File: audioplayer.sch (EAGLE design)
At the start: 28 parts, among them J1 MICRO-SDCARD-CONNECTOR-330006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, J10 CONNECTOR-HEADER-8P-3460290P1, J11 CONNECTOR-HEADER-8P-3460290P1, J2 JST-2P-SMD-PW-3410050P1, J3 MICRO-USB-5P-340015001, J4 CONNECTOR-HEADER-2X3P-3460180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, J5 AUDIO-CONNECTOR-6P-SMD-344003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, J6 SCREW-TERMINAL-2P-3470070P1, J7 CONNECTOR-HEADER-6P-3460650P1, J8 CONNECTOR-HEADER-6P-3460270P1, J9 CONNECTOR-HEADER-10P-3460170P1, K1 BUTTON-4P-3100010P1, U1 ATMEGA328P-AU-1030060P1, U2 CN3065-1320040P1, U3 XC6206-3.3-1300260P1, X1 CRYSTAL-0500290P1

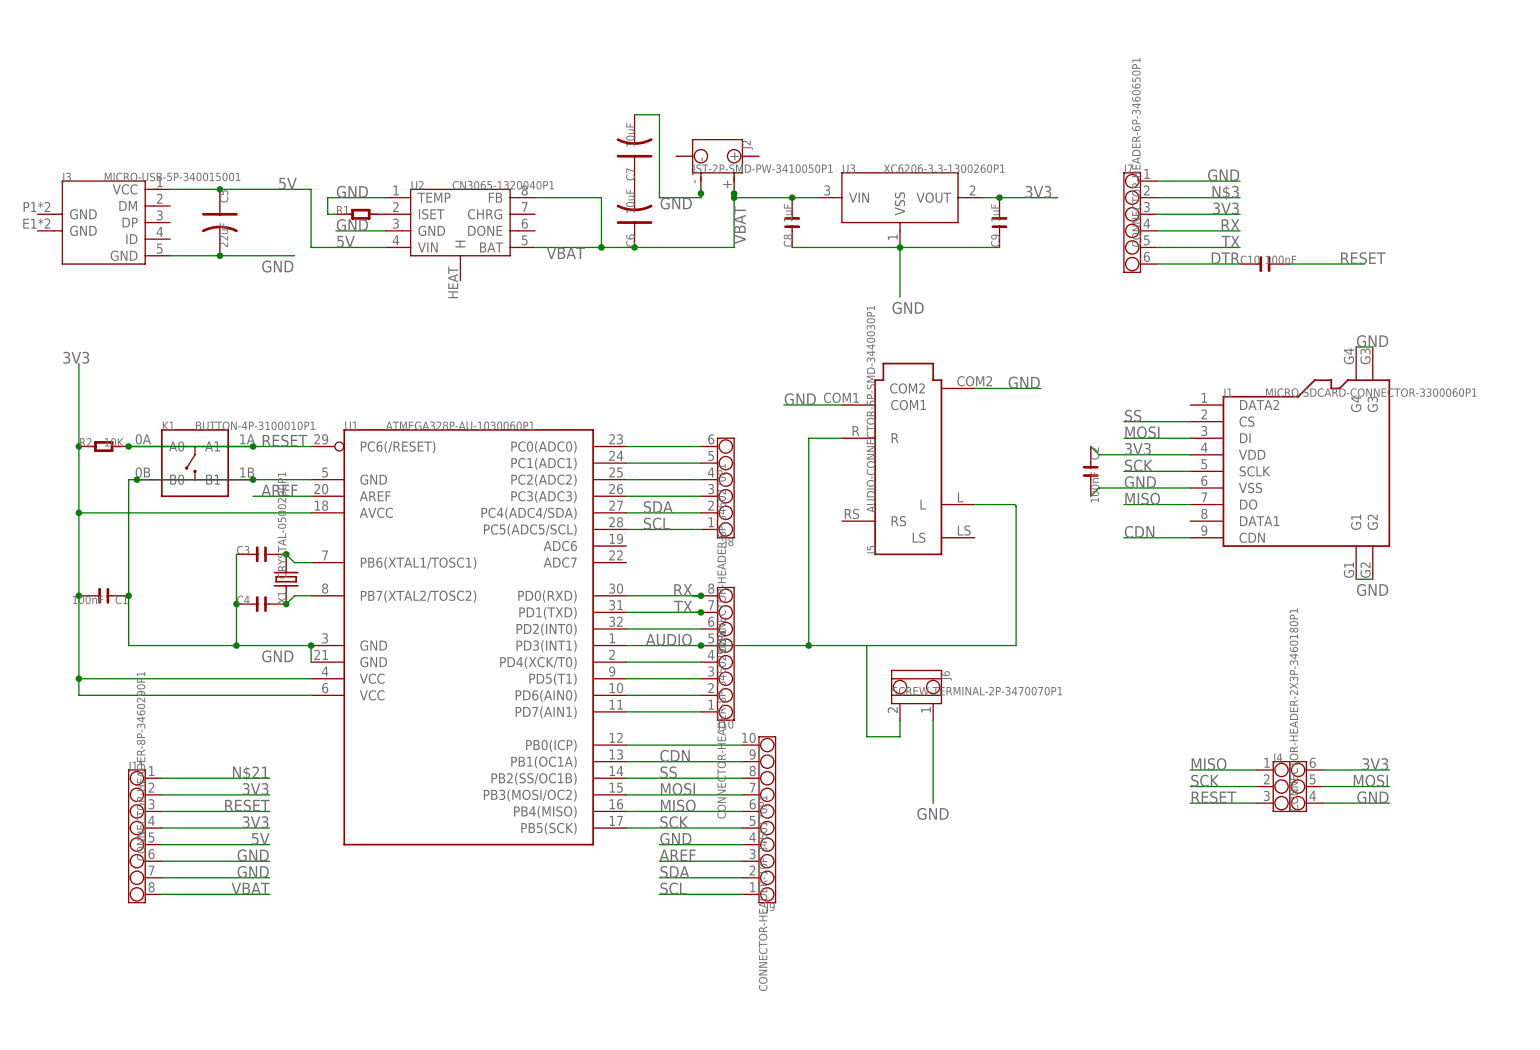
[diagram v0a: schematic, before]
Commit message: 1.5 hrs: routing.
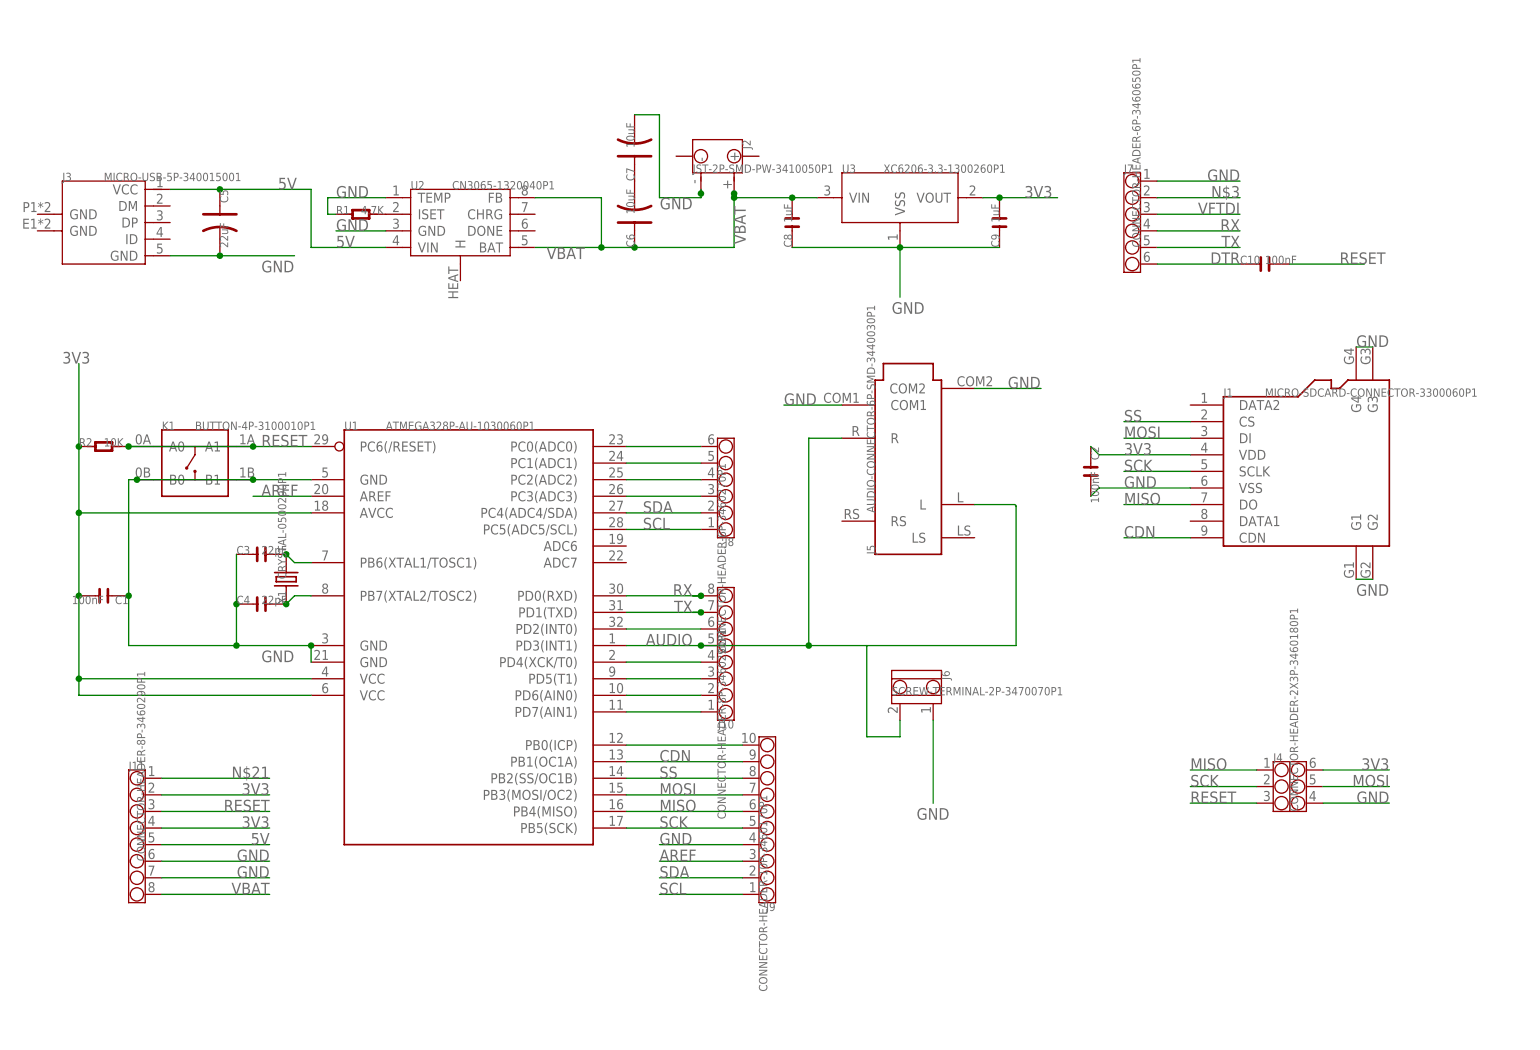
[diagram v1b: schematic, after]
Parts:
- C3, C4: value (none) -> 22pF
- R1: value (none) -> 4.7K
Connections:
- new net VFTDI: J7.3
- net 3V3: no longer J7.3
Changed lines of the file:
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@@
 <setting verticaltext="up"/>
 </settings>
-<grid distance="0.05" unitdist="inch" unit="inch" style="lines" multiple="1" display="no" altdistance="0.01" altunitdist="inch" altunit="inch"/>
+<grid distance="0.1" unitdist="inch" unit="inch" style="lines" multiple="1" display="no" altdistance="0.01" altunitdist="inch" altunit="inch"/>
 <layers>
 <layer number="1" name="Top" color="4" fill="1" visible="no" active="no"/>
@@
 <class number="0" name="default" width="0" drill="0">
 </class>
+<class number="1" name="power" width="0.254" drill="0">
+</class>
 </classes>
 <parts>
@@
 <part name="K1" library="OPL" deviceset="BUTTON-4P" device="-3100010P1"/>
 <part name="X1" library="OPL" deviceset="CRYSTAL*" device="-0500290P1"/>
-<part name="C3" library="OPL" deviceset="C*" device="-0603"/>
-<part name="C4" library="OPL" deviceset="C*" device="-0603"/>
+<part name="C3" library="OPL" deviceset="C*" device="-0603" value="22pF"/>
+<part name="C4" library="OPL" deviceset="C*" device="-0603" value="22pF"/>
 <part name="J5" library="OPL" deviceset="AUDIO-CONNECTOR-6P-SMD" device="-3440030P1"/>
 <part name="C5" library="OPL" deviceset="C-POLAR*" device="-B" value="22uF"/>
@@
 <part name="J7" library="OPL" deviceset="CONNECTOR-HEADER-6P" device="-3460650P1"/>
 <part name="C10" library="OPL" deviceset="C*" device="-0603" value="100nF"/>
-<part name="R1" library="OPL" deviceset="R*" device="-0603"/>
+<part name="R1" library="OPL" deviceset="R*" device="-0603" value="4.7K"/>
 <part name="J8" library="OPL" deviceset="CONNECTOR-HEADER-6P" device="-3460270P1"/>
 <part name="J10" library="OPL" deviceset="CONNECTOR-HEADER-8P" device="-3460290P1"/>
@@
 </busses>
 <nets>
-<net name="3V3" class="0">
+<net name="3V3" class="1">
 <segment>
 <pinref part="U1" gate="U" pin="AVCC"/>
@@
 </segment>
 <segment>
-<pinref part="J7" gate="J" pin="3"/>
-<wire x1="142.24" y1="119.38" x2="154.94" y2="119.38" width="0.1524" layer="91"/>
-<label x="154.94" y="119.38" size="1.778" layer="95" rot="MR0"/>
-</segment>
-<segment>
 <pinref part="J11" gate="J" pin="2"/>
 <wire x1="-10.16" y1="30.48" x2="6.35" y2="30.48" width="0.1524" layer="91"/>
@@
 </segment>
 </net>
-<net name="GND" class="0">
+<net name="GND" class="1">
 <segment>
 <pinref part="U1" gate="U" pin="GND@1"/>
@@
 </segment>
 </net>
-<net name="5V" class="0">
+<net name="5V" class="1">
 <segment>
 <pinref part="J3" gate="USB" pin="VCC"/>
@@
 </segment>
 </net>
-<net name="VBAT" class="0">
+<net name="VBAT" class="1">
 <segment>
 <pinref part="U2" gate="U" pin="BAT"/>
@@
 </segment>
 </net>
+<net name="VFTDI" class="1">
+<segment>
+<pinref part="J7" gate="J" pin="3"/>
+<wire x1="142.24" y1="119.38" x2="154.94" y2="119.38" width="0.1524" layer="91"/>
+<label x="154.94" y="119.38" size="1.778" layer="95" rot="MR0"/>
+</segment>
+</net>
